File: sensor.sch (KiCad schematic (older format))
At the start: 1 part

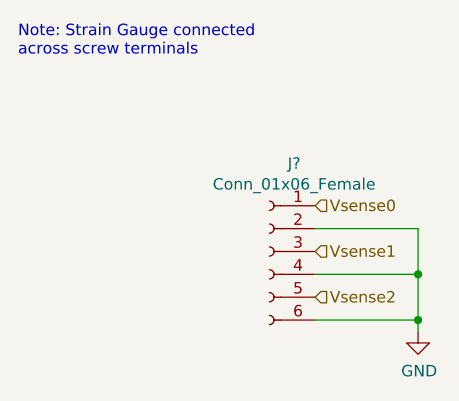
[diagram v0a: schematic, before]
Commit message: left off reworking bottom of board
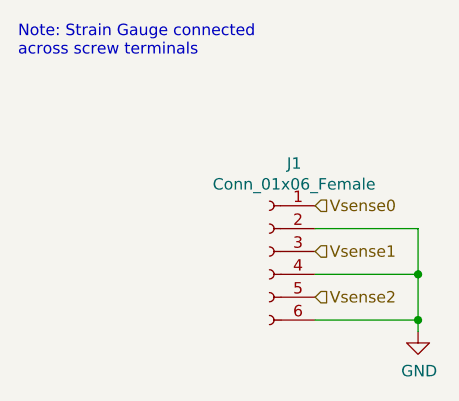
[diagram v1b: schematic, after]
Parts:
- J1: renamed from J?; footprint Connector_Molex:Molex_Pico-Clasp_202396-0607_1x06-1MP_P1.00mm_Horizontal -> Connector_Molex:Molex_PicoBlade_53047-0610_1x06_P1.25mm_Vertical
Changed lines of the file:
@@
 $Descr A4 11693 8268
 encoding utf-8
-Sheet 4 21
+Sheet 3 21
 Title ""
 Date ""
@@
 AR Path="/601B4C19/601A6FD1/60194B46" Ref="#PWR074"  Part="1"
 AR Path="/601B4C19/601A6FD6/60194B46" Ref="#PWR075"  Part="1"
-F 0 "#PWR017" H 5650 4000 50  0001 C CNN
+F 0 "#PWR016" H 5650 4000 50  0001 C CNN
 F 1 "GND" H 5655 4077 50  0000 C CNN
 F 2 "" H 5650 4250 50  0001 C CNN
@@
 U 1 1 60B45C6C
 P 5000 3900
-F 0 "J?" H 4892 4285 50  0000 C CNN
+AR Path="/6017CC5E/6019B999/60B45C6C" Ref="J?"  Part="1"
+AR Path="/6017CC5E/60194350/60B45C6C" Ref="J1"  Part="1"
+AR Path="/601927EB/601A1EA6/60B45C6C" Ref="J2"  Part="1"
+AR Path="/6019C043/601A47AA/60B45C6C" Ref="J3"  Part="1"
+AR Path="/6019DBCE/601A6FCC/60B45C6C" Ref="J4"  Part="1"
+AR Path="/601B4C0E/60194350/60B45C6C" Ref="J5"  Part="1"
+AR Path="/601B4C11/601A1EA6/60B45C6C" Ref="J6"  Part="1"
+AR Path="/601B4C16/601A47AA/60B45C6C" Ref="J7"  Part="1"
+AR Path="/601B4C19/601A6FCC/60B45C6C" Ref="J8"  Part="1"
+AR Path="/601B73B7/60194350/60B45C6C" Ref="J9"  Part="1"
+AR Path="/601B73BA/601A1EA6/60B45C6C" Ref="J10"  Part="1"
+F 0 "J1" H 4892 4285 50  0000 C CNN
 F 1 "Conn_01x06_Female" H 4892 4194 50  0000 C CNN
-F 2 "Connector_Molex:Molex_Pico-Clasp_202396-0607_1x06-1MP_P1.00mm_Horizontal" H 5000 3900 50  0001 C CNN
+F 2 "Connector_Molex:Molex_PicoBlade_53047-0610_1x06_P1.25mm_Vertical" H 5000 3900 50  0001 C CNN
 F 3 "https://www.digikey.com/en/products/detail/molex/5013300600/1531503?s=N4IgjCBcoLQBxVAYygMwIYBsDOBTANCAPZQDaIAnAAxUgC6Avg4QExkgCsVYAzDzQDYa9BkA" H 5000 3900 50  0001 C CNN
 	1    5000 3900
